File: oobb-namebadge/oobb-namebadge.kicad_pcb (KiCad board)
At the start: 2 copper layers, 90 x 70 mm, 26 parts, among them J1 Conn_02x03_Odd_Even, J2 Conn_02x03_Odd_Even, J3 Conn_02x03_Odd_Even, J4 Conn_02x03_Odd_Even, J5 Conn_01x06, J6 Conn_02x03_Odd_Even, J7 Conn_01x01, J8 Conn_01x01, SW1 SW_SPDT, U1 AP1117-15, U2 lipo-charger-boost

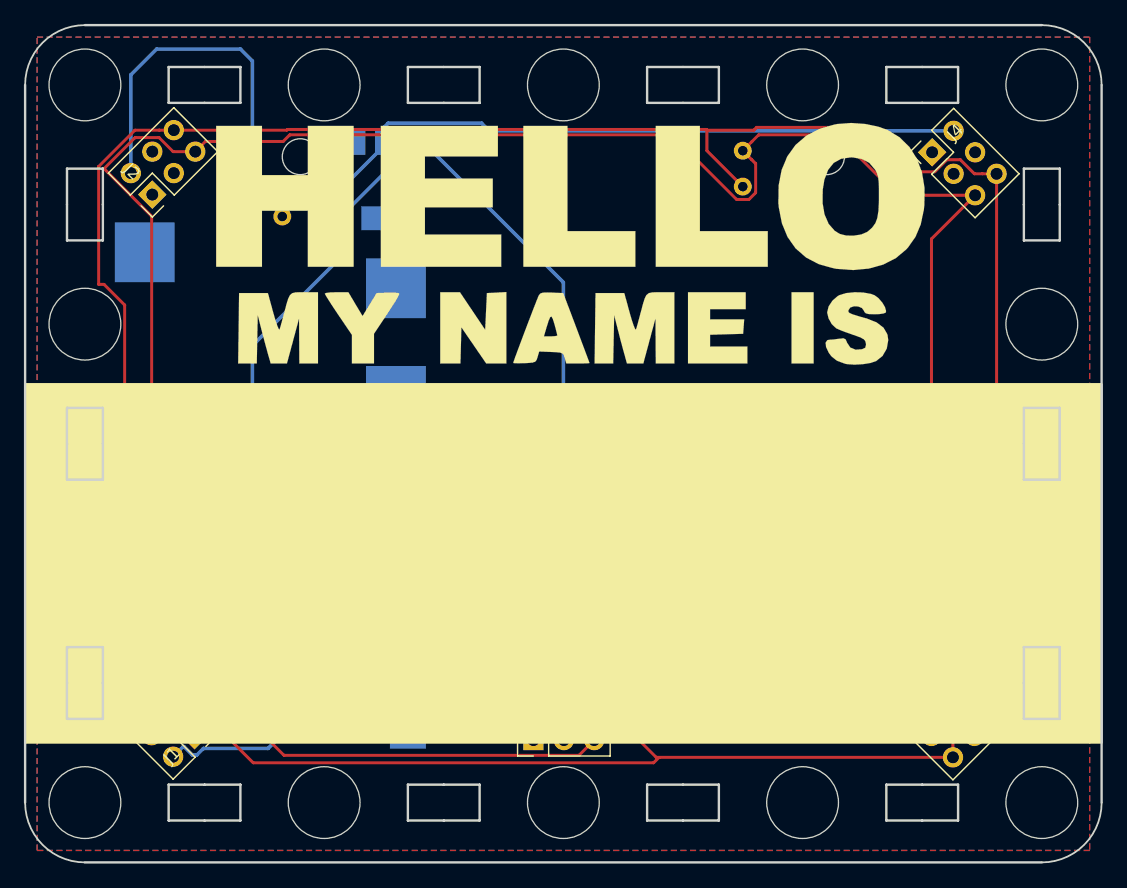
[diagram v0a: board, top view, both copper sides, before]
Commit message: fp files
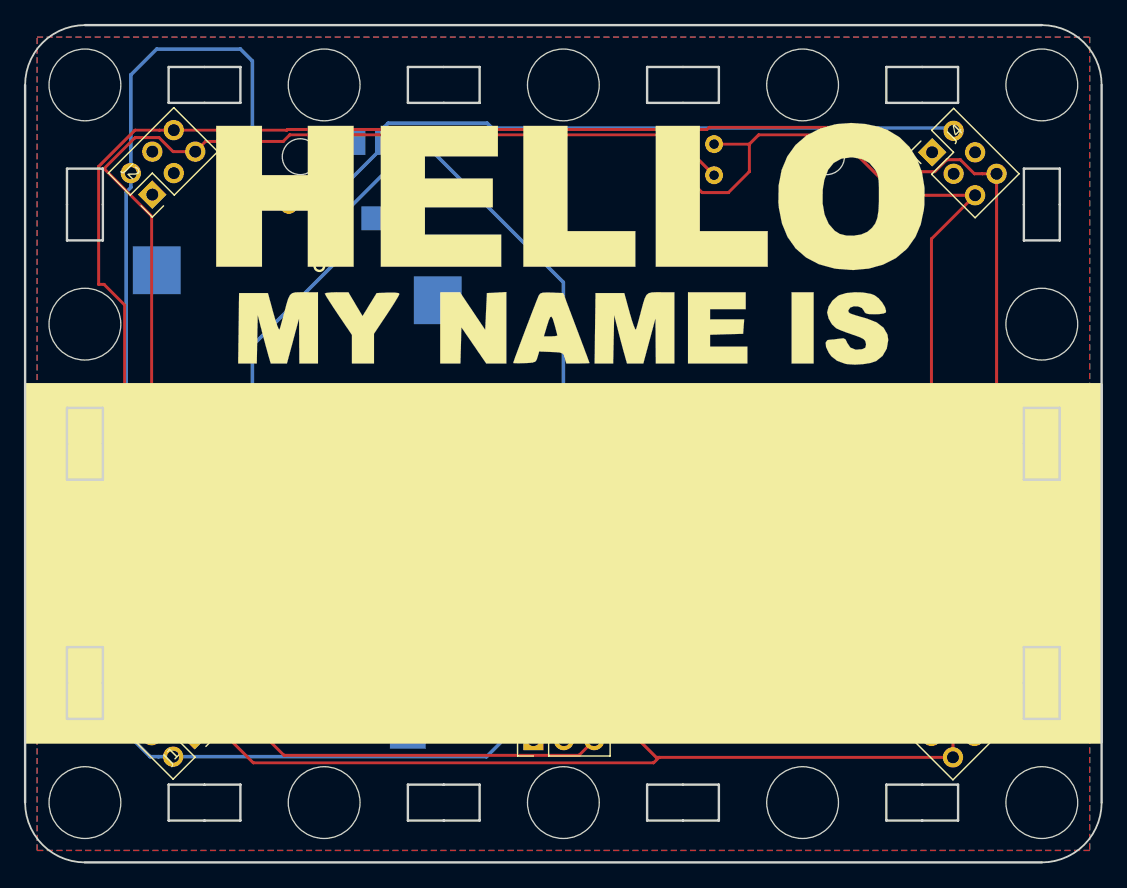
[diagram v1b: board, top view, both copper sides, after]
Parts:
- moved U2 2.06 mm to (141.0, 108.5)
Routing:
- net +3V3: track 173.4 -> 218.6 mm
- net /boost-out: track 87.1 -> 89.4 mm
- net /gpio2: track 251.7 -> 253.3 mm
- net /gpio1: track 262.0 -> 260.9 mm
- net Net-(SW1-Pad2): track 26.1 -> 27.2 mm
